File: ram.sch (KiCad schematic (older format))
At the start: 8 parts, among them U1 LFE5U-85F-6BG381C, U2 IS42S16320D-6BLI

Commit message: Adding DDR3 symbol and footprint
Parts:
- removed U2: IS42S16320D-6BLI, IS42S16320D:IS42S16320D-6BLI, symbol mt48lc16m16a2tg:IS42S16320D-6BLI
- added U2: MT41K256M16TW-107_P, MT41K256M16TW-107_P:BGA96C80P9X16_800X1400X120, symbol MT41K256M16TW-107_P:MT41K256M16TW-107_P
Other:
- moved on the sheet: C16, C33, C34, C35, C52

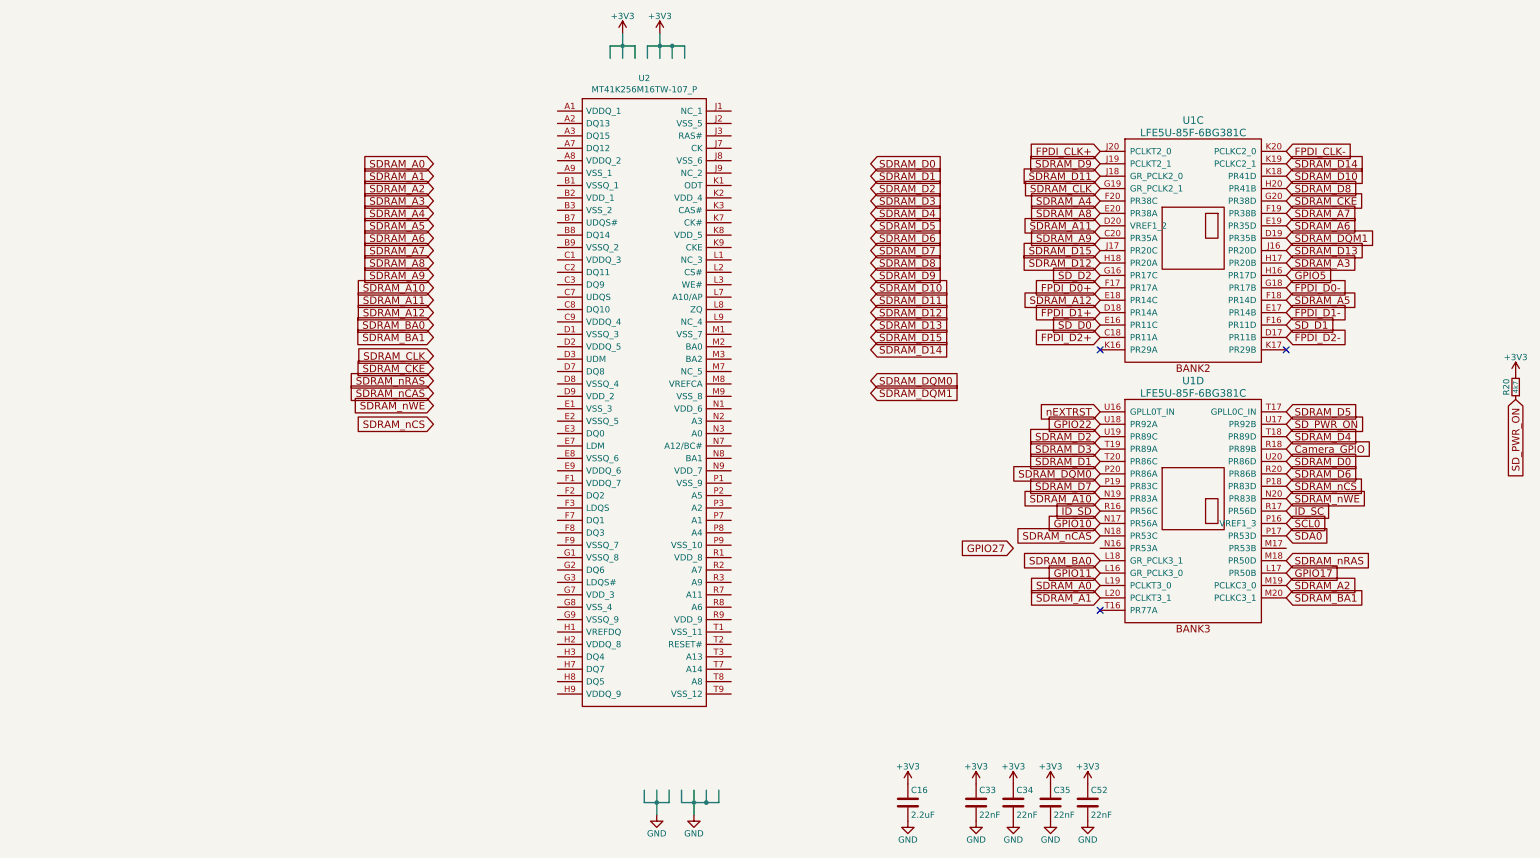
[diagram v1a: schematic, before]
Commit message: Adding ecp5-dc-scm ddr3 schematics and footprint
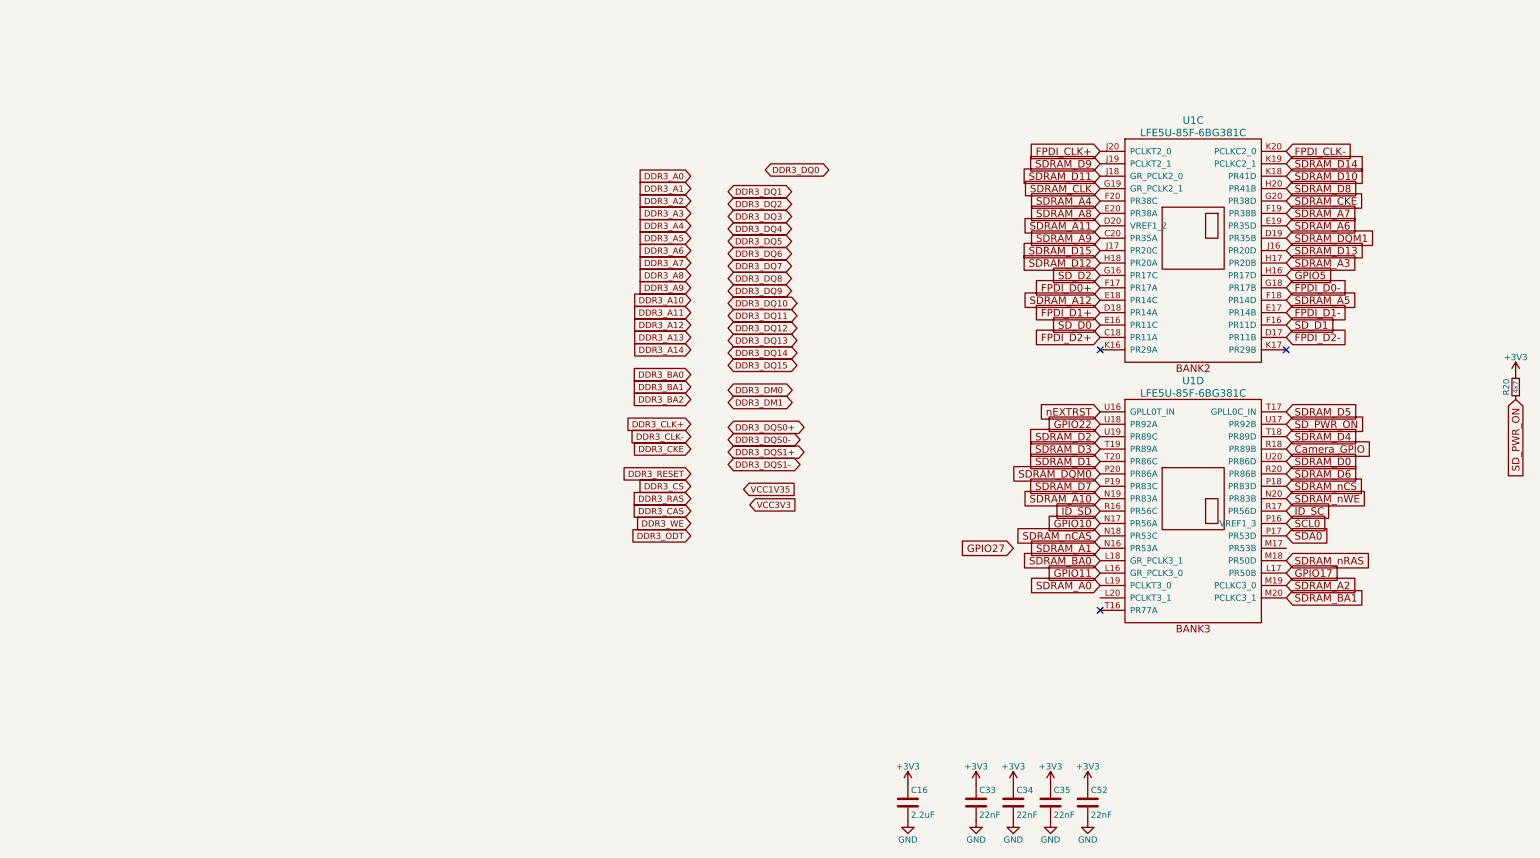
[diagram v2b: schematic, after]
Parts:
- removed U2: MT41K256M16TW-107_P, MT41K256M16TW-107_P:BGA96C80P9X16_800X1400X120, symbol MT41K256M16TW-107_P:MT41K256M16TW-107_P
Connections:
- net labels added: DDR3_A0, DDR3_A1, DDR3_A10, DDR3_A11, DDR3_A12, DDR3_A13, DDR3_A14, DDR3_A2, DDR3_A3, DDR3_A4, DDR3_A5, DDR3_A6, DDR3_A7, DDR3_A8, DDR3_A9, DDR3_BA0, DDR3_BA1, DDR3_BA2, DDR3_CAS, DDR3_CKE, DDR3_CLK+, DDR3_CLK-, DDR3_CS, DDR3_DM0, DDR3_DM1, DDR3_DQ0, DDR3_DQ1, DDR3_DQ10, DDR3_DQ11, DDR3_DQ12, DDR3_DQ13, DDR3_DQ14, DDR3_DQ15, DDR3_DQ2, DDR3_DQ3, DDR3_DQ4, DDR3_DQ5, DDR3_DQ6, DDR3_DQ7, DDR3_DQ8, DDR3_DQ9, DDR3_DQS0+, DDR3_DQS0-, DDR3_DQS1+, DDR3_DQS1-, DDR3_ODT, DDR3_RAS, DDR3_RESET, DDR3_WE, VCC1V35, VCC3V3
- wire segments 28 -> 0

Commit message: DDR3 GND and VCC
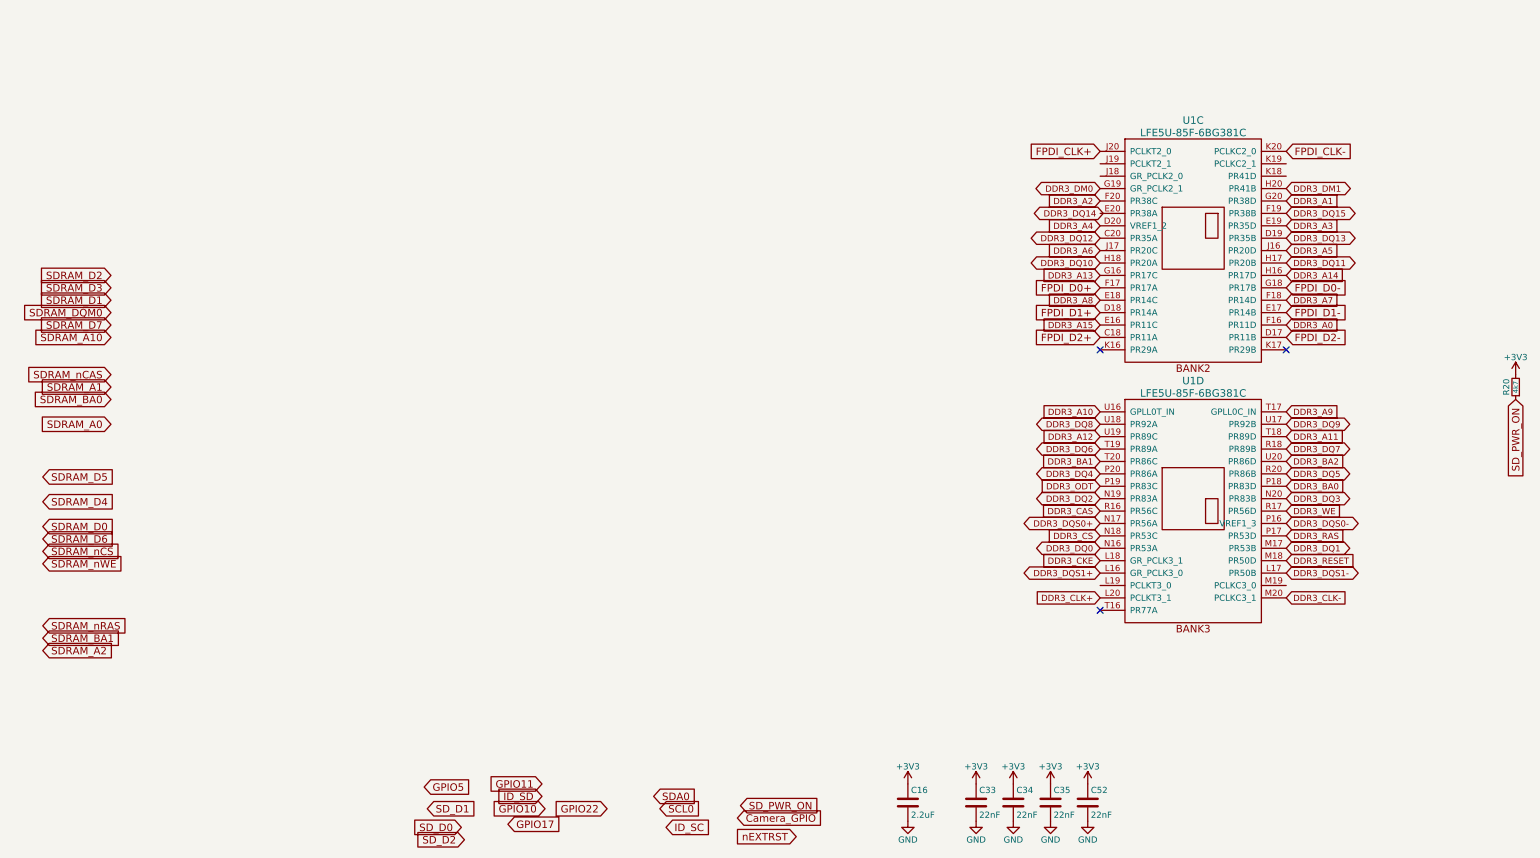
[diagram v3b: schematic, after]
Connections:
- net SDRAM_A11 is gone; now on net DDR3_A4: U1.D20 (VREF1_2)
- net SDRAM_A12 is gone; now on net DDR3_A8: U1.E18 (PR14C)
- net SDRAM_A3 is gone; now on net DDR3_DQ11: U1.H17 (PR20B)
- net SDRAM_A4 is gone; now on net DDR3_A2: U1.F20 (PR38C)
- net SDRAM_A5 is gone; now on net DDR3_A7: U1.F18 (PR14D)
- net SDRAM_A6 is gone; now on net DDR3_A3: U1.E19 (PR35D)
- net SDRAM_A7 is gone; now on net DDR3_DQ15: U1.F19 (PR38B)
- net SDRAM_A9 is gone; now on net DDR3_DQ12: U1.C20 (PR35A)
- net SDRAM_CKE is gone; now on net DDR3_A1: U1.G20 (PR38D)
- net SDRAM_CLK is gone; now on net DDR3_DM0: U1.G19 (GR_PCLK2_1)
- net SDRAM_D12 is gone; now on net DDR3_DQ10: U1.H18 (PR20A)
- net SDRAM_D13 is gone; now on net DDR3_A5: U1.J16 (PR20D)
- net SDRAM_D15 is gone; now on net DDR3_A6: U1.J17 (PR20C)
- net SDRAM_D8 is gone; now on net DDR3_DM1: U1.H20 (PR41B)
- net SDRAM_DQM1 is gone; now on net DDR3_DQ13: U1.D19 (PR35B)
- net Camera_GPIO: no longer U1.R18 (PR89B)
- net DDR3_A0: now also U1.F16 (PR11D)
- net DDR3_A10: now also U1.U16 (GPLL0T_IN)
- net DDR3_A11: now also U1.T18 (PR89D)
- net DDR3_A12: now also U1.U19 (PR89C)
- net DDR3_A13: now also U1.G16 (PR17C)
- net DDR3_A14: now also U1.H16 (PR17D)
- net DDR3_A9: now also U1.T17 (GPLL0C_IN)
- net DDR3_BA0: now also U1.P18 (PR83D)
- net DDR3_BA1: now also U1.T20 (PR86C)
- net DDR3_BA2: now also U1.U20 (PR86D)
- net DDR3_CAS: now also U1.R16 (PR56C)
- net DDR3_CKE: now also U1.L18 (GR_PCLK3_1)
- net DDR3_CLK+: now also U1.L20 (PCLKT3_1)
- net DDR3_CLK-: now also U1.M20 (PCLKC3_1)
- net DDR3_CS: now also U1.N18 (PR53C)
- net DDR3_DQ0: now also U1.N16 (PR53A)
- net DDR3_DQ1: now also U1.M17 (PR53B)
- net DDR3_DQ2: now also U1.N19 (PR83A)
- net DDR3_DQ3: now also U1.N20 (PR83B)
- net DDR3_DQ4: now also U1.P20 (PR86A)
- net DDR3_DQ5: now also U1.R20 (PR86B)
- net DDR3_DQ6: now also U1.T19 (PR89A)
- net DDR3_DQ7: now also U1.R18 (PR89B)
- net DDR3_DQ8: now also U1.U18 (PR92A)
- net DDR3_DQ9: now also U1.U17 (PR92B)
- net DDR3_DQS0+: now also U1.N17 (PR56A)
- net DDR3_DQS0-: now also U1.P16 (VREF1_3)
- net DDR3_DQS1+: now also U1.L16 (GR_PCLK3_0)
- net DDR3_DQS1-: now also U1.L17 (PR50B)
- net DDR3_ODT: now also U1.P19 (PR83C)
- net DDR3_RAS: now also U1.P17 (PR53D)
- net DDR3_RESET: now also U1.M18 (PR50D)
- net DDR3_WE: now also U1.R17 (PR56D)
- net GPIO10: no longer U1.N17 (PR56A)
- net GPIO11: no longer U1.L16 (GR_PCLK3_0)
- net GPIO17: no longer U1.L17 (PR50B)
- net GPIO22: no longer U1.U18 (PR92A)
- net GPIO5: no longer U1.H16 (PR17D)
- net ID_SC: no longer U1.R17 (PR56D)
- net ID_SD: no longer U1.R16 (PR56C)
- net SCL0: no longer U1.P16 (VREF1_3)
- net SDA0: no longer U1.P17 (PR53D)
- net SDRAM_A0: no longer U1.L19 (PCLKT3_0)
- net SDRAM_A1: no longer U1.N16 (PR53A)
- net SDRAM_A10: no longer U1.N19 (PR83A)
- net SDRAM_A2: no longer U1.M19 (PCLKC3_0)
- net SDRAM_BA0: no longer U1.L18 (GR_PCLK3_1)
- net SDRAM_BA1: no longer U1.M20 (PCLKC3_1)
- net SDRAM_D0: no longer U1.U20 (PR86D)
- net SDRAM_D1: no longer U1.T20 (PR86C)
- net SDRAM_D2: no longer U1.U19 (PR89C)
- net SDRAM_D3: no longer U1.T19 (PR89A)
- net SDRAM_D4: no longer U1.T18 (PR89D)
- net SDRAM_D5: no longer U1.T17 (GPLL0C_IN)
- net SDRAM_D6: no longer U1.R20 (PR86B)
- net SDRAM_D7: no longer U1.P19 (PR83C)
- net SDRAM_DQM0: no longer U1.P20 (PR86A)
- net SDRAM_nCAS: no longer U1.N18 (PR53C)
- net SDRAM_nCS: no longer U1.P18 (PR83D)
- net SDRAM_nRAS: no longer U1.M18 (PR50D)
- net SDRAM_nWE: no longer U1.N20 (PR83B)
- net SD_D0: no longer U1.E16 (PR11C)
- net SD_D1: no longer U1.F16 (PR11D)
- net SD_D2: no longer U1.G16 (PR17C)
- net SD_PWR_ON: no longer U1.U17 (PR92B)
- net nEXTRST: no longer U1.U16 (GPLL0T_IN)
- net SDRAM_A8: no longer names the net of U1.E20 (PR38A)
- net SDRAM_D10: no longer names the net of U1.K18 (PR41D)
- net SDRAM_D11: no longer names the net of U1.J18 (GR_PCLK2_0)
- net SDRAM_D14: no longer names the net of U1.K19 (PCLKC2_1)
- net SDRAM_D9: no longer names the net of U1.J19 (PCLKT2_1)
- new net DDR3_A15: U1.E16 (PR11C)
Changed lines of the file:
@@
 Comment4 ""
 $EndDescr
-Text GLabel 8100 4200 2    60   Input ~ 0
+Text GLabel -1925 4725 2    60   Input ~ 0
 SDRAM_D0
-Text GLabel 6600 4200 0    60   Input ~ 0
+Text GLabel -1375 2900 0    60   Input ~ 0
 SDRAM_D1
-Text GLabel 6600 4000 0    60   Input ~ 0
+Text GLabel -1375 2700 0    60   Input ~ 0
 SDRAM_D2
-Text GLabel 6600 4100 0    60   Input ~ 0
+Text GLabel -1375 2800 0    60   Input ~ 0
 SDRAM_D3
-Text GLabel 8100 4000 2    60   Input ~ 0
+Text GLabel -1925 4525 2    60   Input ~ 0
 SDRAM_D4
-Text GLabel 8100 3800 2    60   Input ~ 0
+Text GLabel -1925 4325 2    60   Input ~ 0
 SDRAM_D5
-Text GLabel 8100 4300 2    60   Input ~ 0
+Text GLabel -1925 4825 2    60   Input ~ 0
 SDRAM_D6
-Text GLabel 6600 4400 0    60   Input ~ 0
+Text GLabel -1375 3100 0    60   Input ~ 0
 SDRAM_D7
-Text GLabel 8100 2000 2    60   Input ~ 0
-SDRAM_D8
-Text GLabel 8100 1900 2    60   Input ~ 0
-SDRAM_D10
-Text GLabel 8100 2500 2    60   Input ~ 0
-SDRAM_D13
-Text GLabel 8100 1800 2    60   Input ~ 0
-SDRAM_D14
-Text GLabel 8100 2600 2    60   Input ~ 0
-SDRAM_A3
-Text GLabel 8100 2900 2    60   Input ~ 0
-SDRAM_A5
-Text GLabel 8100 2300 2    60   Input ~ 0
-SDRAM_A6
-Text GLabel 8100 2200 2    60   Input ~ 0
-SDRAM_A7
-Text GLabel 6600 4500 0    60   Input ~ 0
+Text GLabel -1375 3200 0    60   Input ~ 0
 SDRAM_A10
-Text GLabel 6600 5000 0    60   Input ~ 0
+Text GLabel -1375 3700 0    60   Input ~ 0
 SDRAM_BA0
-Text GLabel 8100 2100 2    60   Input ~ 0
-SDRAM_CKE
-Text GLabel 6600 4300 0    60   Input ~ 0
+Text GLabel -1375 3000 0    60   Input ~ 0
 SDRAM_DQM0
-Text GLabel 8100 2400 2    60   Input ~ 0
-SDRAM_DQM1
-Text GLabel 8100 5000 2    60   Input ~ 0
+Text GLabel -1925 5525 2    60   Input ~ 0
 SDRAM_nRAS
-Text GLabel 6600 4800 0    60   Input ~ 0
+Text GLabel -1375 3500 0    60   Input ~ 0
 SDRAM_nCAS
-Text GLabel 8100 4500 2    60   Input ~ 0
+Text GLabel -1925 5025 2    60   Input ~ 0
 SDRAM_nWE
-Text GLabel 8100 4400 2    60   Input ~ 0
+Text GLabel -1925 4925 2    60   Input ~ 0
 SDRAM_nCS
 $Comp
@@
 Text GLabel 8100 1700 2    60   Input ~ 0
 FPDI_CLK-
-Text GLabel 8100 2700 2    60   Input ~ 0
+Text GLabel 1150 6825 2    60   Input ~ 0
 GPIO5
 Text GLabel 9950 3700 3    60   Input ~ 0
@@
 	-1   0    0    1
 $EndComp
-Text GLabel 6600 2700 0    60   Input ~ 0
+Text GLabel 1475 7250 0    60   Input ~ 0
 SD_D2
-Text GLabel 3300 1900 0    50   Input ~ 0
+Text GLabel 8100 3100 2    50   Input ~ 0
 DDR3_A0
-Text GLabel 3300 2000 0    50   Input ~ 0
+Text GLabel 8100 2100 2    50   Input ~ 0
 DDR3_A1
-Text GLabel 3300 2100 0    50   Input ~ 0
+Text GLabel 6600 2100 0    50   Input ~ 0
 DDR3_A2
-Text GLabel 3300 2200 0    50   Input ~ 0
+Text GLabel 8100 2300 2    50   Input ~ 0
 DDR3_A3
-Text GLabel 3300 2300 0    50   Input ~ 0
+Text GLabel 6600 2300 0    50   Input ~ 0
 DDR3_A4
-Text GLabel 3300 2400 0    50   Input ~ 0
+Text GLabel 8100 2500 2    50   Input ~ 0
 DDR3_A5
-Text GLabel 3300 2500 0    50   Input ~ 0
+Text GLabel 6600 2500 0    50   Input ~ 0
 DDR3_A6
-Text GLabel 3300 2600 0    50   Input ~ 0
+Text GLabel 8100 2900 2    50   Input ~ 0
 DDR3_A7
-Text GLabel 3300 2700 0    50   Input ~ 0
+Text GLabel 6600 2900 0    50   Input ~ 0
 DDR3_A8
-Text GLabel 3300 2800 0    50   Input ~ 0
+Text GLabel 8100 3800 2    50   Input ~ 0
 DDR3_A9
-Text GLabel 3300 2900 0    50   Input ~ 0
+Text GLabel 6600 3800 0    50   Input ~ 0
 DDR3_A10
-Text GLabel 3300 3000 0    50   Input ~ 0
+Text GLabel 8100 4000 2    50   Input ~ 0
 DDR3_A11
-Text GLabel 3300 3100 0    50   Input ~ 0
+Text GLabel 6600 4000 0    50   Input ~ 0
 DDR3_A12
-Text GLabel 3300 3200 0    50   Input ~ 0
+Text GLabel 6600 2700 0    50   Input ~ 0
 DDR3_A13
-Text GLabel 3300 3300 0    50   Input ~ 0
+Text GLabel 8100 2700 2    50   Input ~ 0
 DDR3_A14
-Text GLabel 3300 3500 0    50   Input ~ 0
+Text GLabel 8100 4400 2    50   Input ~ 0
 DDR3_BA0
-Text GLabel 3300 3600 0    50   Input ~ 0
+Text GLabel 6600 4200 0    50   Input ~ 0
 DDR3_BA1
-Text GLabel 3300 3700 0    50   Input ~ 0
+Text GLabel 8100 4200 2    50   Input ~ 0
 DDR3_BA2
-Text GLabel 3300 3900 0    50   Input ~ 0
+Text GLabel 6600 5300 0    50   Input ~ 0
 DDR3_CLK+
-Text GLabel 3300 4000 0    50   Input ~ 0
+Text GLabel 8100 5300 2    50   Input ~ 0
 DDR3_CLK-
-Text GLabel 3300 4100 0    50   Input ~ 0
+Text GLabel 6600 5000 0    50   Input ~ 0
 DDR3_CKE
-Text GLabel 3300 4300 0    50   Input ~ 0
+Text GLabel 8100 5000 2    50   Input ~ 0
 DDR3_RESET
-Text GLabel 3300 4400 0    50   Input ~ 0
+Text GLabel 6600 4800 0    50   Input ~ 0
 DDR3_CS
-Text GLabel 3300 4600 0    50   Input ~ 0
+Text GLabel 6600 4600 0    50   Input ~ 0
 DDR3_CAS
-Text GLabel 3300 4500 0    50   Input ~ 0
+Text GLabel 8100 4800 2    50   Input ~ 0
 DDR3_RAS
-Text GLabel 3300 4700 0    50   Input ~ 0
+Text GLabel 8100 4600 2    50   Input ~ 0
 DDR3_WE
-Text GLabel 3300 4800 0    50   Input ~ 0
+Text GLabel 6600 4400 0    50   Input ~ 0
 DDR3_ODT
-Text GLabel 3900 1850 2    50   BiDi ~ 0
+Text GLabel 6600 4900 0    50   BiDi ~ 0
 DDR3_DQ0
-Text GLabel 3600 2025 2    50   BiDi ~ 0
+Text GLabel 8100 4900 2    50   BiDi ~ 0
 DDR3_DQ1
-Text GLabel 3600 2125 2    50   BiDi ~ 0
+Text GLabel 6600 4500 0    50   BiDi ~ 0
 DDR3_DQ2
-Text GLabel 3600 2225 2    50   BiDi ~ 0
+Text GLabel 8100 4500 2    50   BiDi ~ 0
 DDR3_DQ3
-Text GLabel 3600 2325 2    50   BiDi ~ 0
+Text GLabel 6600 4300 0    50   BiDi ~ 0
 DDR3_DQ4
-Text GLabel 3600 2425 2    50   BiDi ~ 0
+Text GLabel 8100 4300 2    50   BiDi ~ 0
 DDR3_DQ5
-Text GLabel 3600 2525 2    50   BiDi ~ 0
+Text GLabel 6600 4100 0    50   BiDi ~ 0
 DDR3_DQ6
-Text GLabel 3600 2625 2    50   BiDi ~ 0
+Text GLabel 8100 4100 2    50   BiDi ~ 0
 DDR3_DQ7
-Text GLabel 3600 2725 2    50   BiDi ~ 0
+Text GLabel 6600 3900 0    50   BiDi ~ 0
 DDR3_DQ8
-Text GLabel 3600 2825 2    50   BiDi ~ 0
+Text GLabel 8100 3900 2    50   BiDi ~ 0
 DDR3_DQ9
-Text GLabel 3600 2925 2    50   BiDi ~ 0
+Text GLabel 6600 2600 0    50   BiDi ~ 0
 DDR3_DQ10
-Text GLabel 3600 3025 2    50   BiDi ~ 0
+Text GLabel 8100 2600 2    50   BiDi ~ 0
 DDR3_DQ11
-Text GLabel 3600 3125 2    50   BiDi ~ 0
+Text GLabel 6600 2400 0    50   BiDi ~ 0
 DDR3_DQ12
-Text GLabel 3600 3225 2    50   BiDi ~ 0
+Text GLabel 8100 2400 2    50   BiDi ~ 0
 DDR3_DQ13
-Text GLabel 3600 3325 2    50   BiDi ~ 0
+Text GLabel 6625 2200 0    50   BiDi ~ 0
 DDR3_DQ14
-Text GLabel 3600 3425 2    50   BiDi ~ 0
+Text GLabel 8100 2200 2    50   BiDi ~ 0
 DDR3_DQ15
-Text GLabel 3600 3625 2    50   BiDi ~ 0
+Text GLabel 6600 2000 0    50   BiDi ~ 0
 DDR3_DM0
-Text GLabel 3600 3725 2    50   BiDi ~ 0
+Text GLabel 8100 2000 2    50   BiDi ~ 0
 DDR3_DM1
-Text GLabel 3600 3925 2    50   BiDi ~ 0
+Text GLabel 6600 4700 0    50   BiDi ~ 0
 DDR3_DQS0+
-Text GLabel 3600 4025 2    50   BiDi ~ 0
+Text GLabel 8100 4700 2    50   BiDi ~ 0
 DDR3_DQS0-
-Text GLabel 3600 4125 2    50   BiDi ~ 0
+Text GLabel 6600 5100 0    50   BiDi ~ 0
 DDR3_DQS1+
-Text GLabel 3600 4225 2    50   BiDi ~ 0
+Text GLabel 8100 5100 2    50   BiDi ~ 0
 DDR3_DQS1-
-Text GLabel 3725 4425 2    50   Input ~ 0
-VCC1V35
-Text GLabel 3775 4550 2    50   Input ~ 0
-VCC3V3
-Text GLabel 6600 2900 0    60   Input ~ 0
-SDRAM_A12
-Text GLabel 6600 2000 0    60   Input ~ 0
-SDRAM_CLK
-Text GLabel 6600 2300 0    60   Input ~ 0
-SDRAM_A11
-Text GLabel 6600 2400 0    60   Input ~ 0
-SDRAM_A9
-Text GLabel 6600 2200 0    60   Input ~ 0
-SDRAM_A8
-Text GLabel 6600 2100 0    60   Input ~ 0
-SDRAM_A4
-Text GLabel 6600 2500 0    60   Input ~ 0
-SDRAM_D15
-Text GLabel 6600 2600 0    60   Input ~ 0
-SDRAM_D12
-Text GLabel 6600 1900 0    60   Input ~ 0
-SDRAM_D11
-Text GLabel 6600 1800 0    60   Input ~ 0
-SDRAM_D9
-Text GLabel 8100 3100 2    60   Input ~ 0
+Text GLabel 1175 7000 2    60   Input ~ 0
 SD_D1
-Text GLabel 6600 3100 0    60   Input ~ 0
+Text GLabel 1450 7150 0    60   Input ~ 0
 SD_D0
-Text GLabel 6600 4700 0    60   Input ~ 0
+Text GLabel 2100 6900 0    60   Input ~ 0
+ID_SD
+Text GLabel 4150 7225 0    60   Input ~ 0
+nEXTRST
+Text GLabel 2625 7000 0    60   Input ~ 0
+GPIO22
+Text GLabel 3700 6975 2    60   Input ~ 0
+SD_PWR_ON
+Text GLabel 3675 7075 2    60   Input ~ 0
+Camera_GPIO
+Text GLabel 3100 7150 2    60   Input ~ 0
+ID_SC
+Text GLabel 3050 7000 2    60   Input ~ 0
+SCL0
+Text GLabel 3000 6900 2    60   Input ~ 0
+SDA0
+Text GLabel -1925 5625 2    60   Input ~ 0
+SDRAM_BA1
+Text GLabel -1925 5725 2    60   Input ~ 0
+SDRAM_A2
+Text GLabel -1375 3900 0    60   Input ~ 0
+SDRAM_A0
+Text GLabel 1825 7125 2    60   Input ~ 0
+GPIO17
+Text GLabel -1375 3600 0    60   Input ~ 0
+SDRAM_A1
+Text GLabel 2100 6800 0    60   Input ~ 0
+GPIO11
+Text GLabel 2125 7000 0    60   Input ~ 0
 GPIO10
-Text GLabel 6600 4600 0    60   Input ~ 0
-ID_SD
-Text GLabel 6600 3800 0    60   Input ~ 0
-nEXTRST
-Text GLabel 6600 3900 0    60   Input ~ 0
-GPIO22
-Text GLabel 8100 3900 2    60   Input ~ 0
-SD_PWR_ON
-Text GLabel 8100 4100 2    60   Input ~ 0
-Camera_GPIO
-Text GLabel 8100 4600 2    60   Input ~ 0
-ID_SC
-Text GLabel 8100 4700 2    60   Input ~ 0
-SCL0
-Text GLabel 8100 4800 2    60   Input ~ 0
-SDA0
-Text GLabel 8100 5300 2    60   Input ~ 0
-SDRAM_BA1
-Text GLabel 8100 5200 2    60   Input ~ 0
-SDRAM_A2
-Text GLabel 6600 5200 0    60   Input ~ 0
-SDRAM_A0
-Text GLabel 5900 4900 0    60   Input ~ 0
-GPIO27
-Text GLabel 8100 5100 2    60   Input ~ 0
-GPIO17
-Text GLabel 6600 5100 0    60   Input ~ 0
-GPIO11
-Text GLabel 6600 4900 0    60   Input ~ 0
-SDRAM_A1
+Text GLabel 6600 3100 0    50   Input ~ 0
+DDR3_A15
 $EndSCHEMATC
